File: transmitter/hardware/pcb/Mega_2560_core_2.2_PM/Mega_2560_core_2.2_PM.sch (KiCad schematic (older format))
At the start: 0 parts

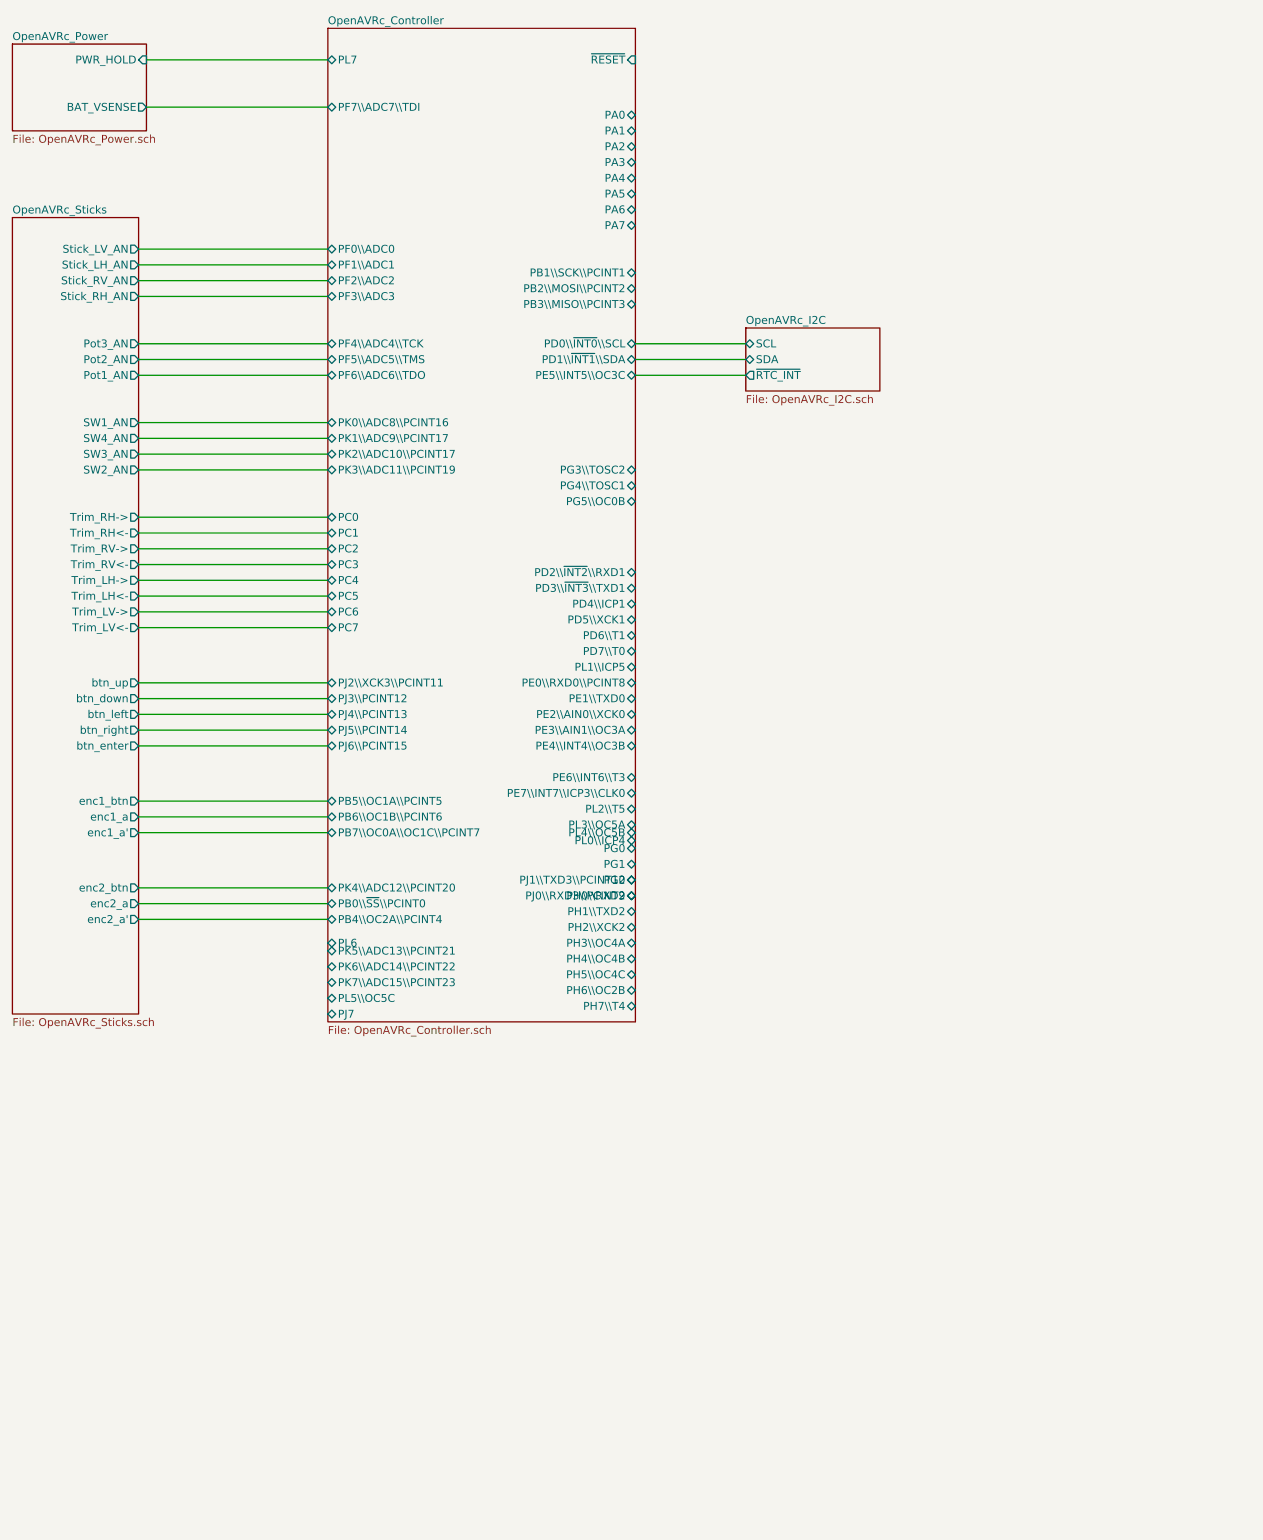
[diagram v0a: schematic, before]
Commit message: WIP commit
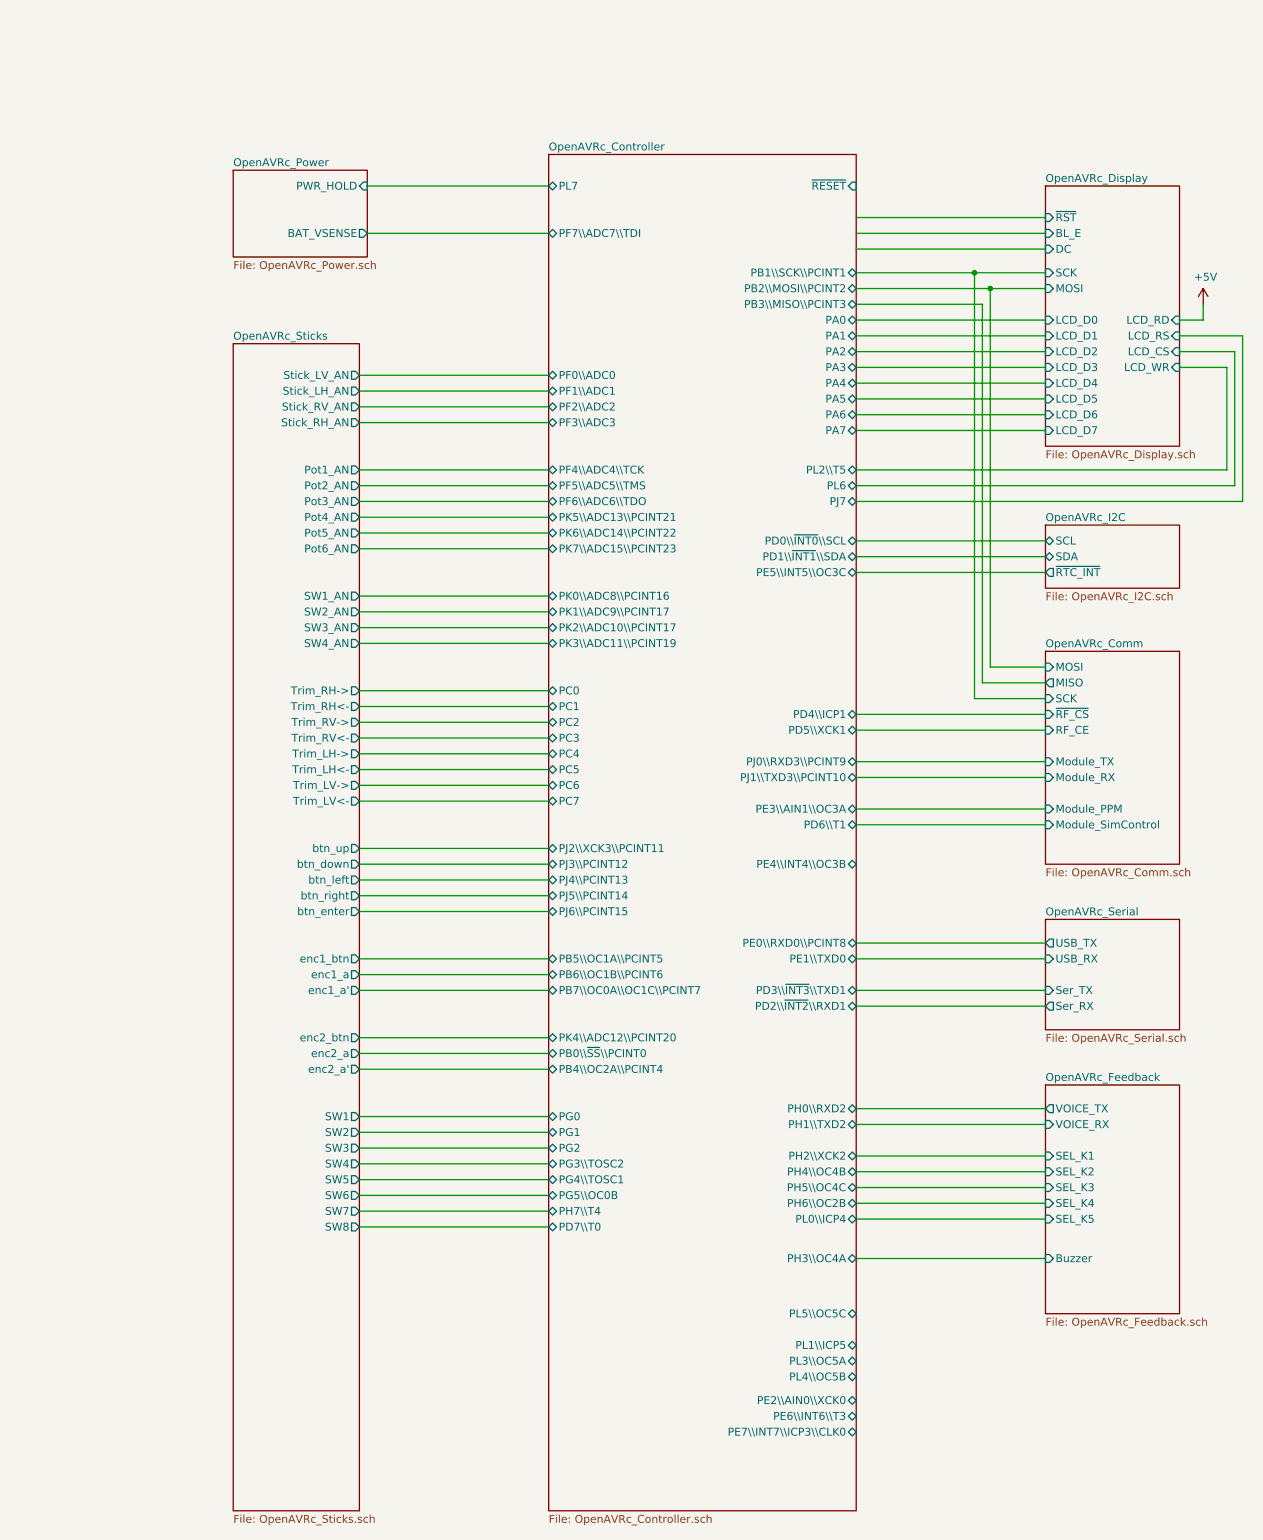
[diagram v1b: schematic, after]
